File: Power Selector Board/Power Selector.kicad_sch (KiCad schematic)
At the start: 23 parts, among them J101 MSD-DB01M-12P, J102 MSD-DB01F-12P_1, J103 64900221122, J104 64900221122, J105 64900221122, K101 G6SK-2G DC24, U101 1720466, U102 LMW78_24-0.3RL, U103 LMW78_24-0.3RL

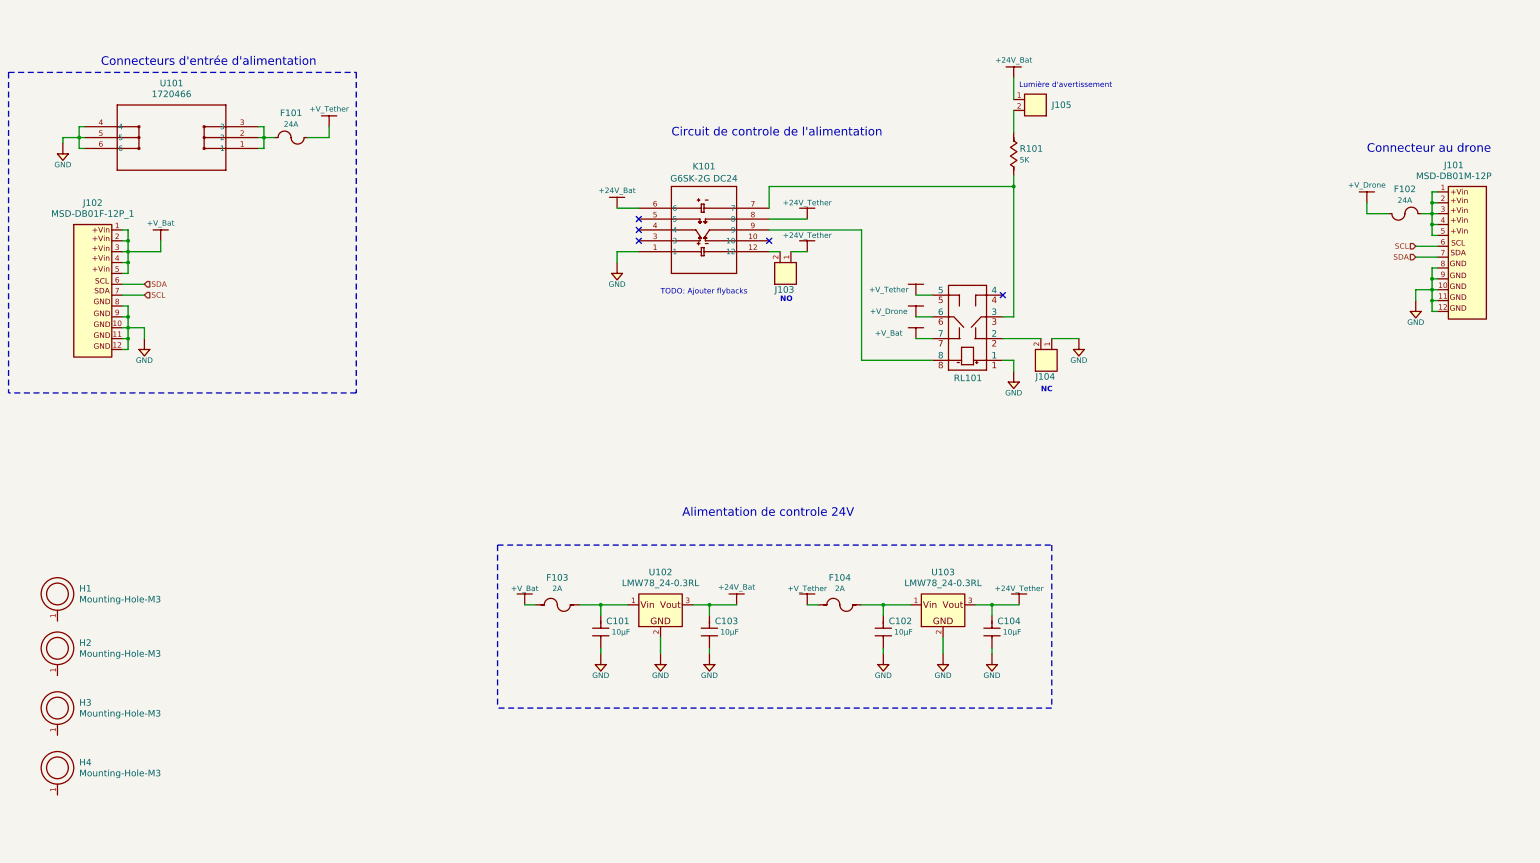
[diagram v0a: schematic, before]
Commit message: Fix du bug github, devrait etre la bonne version
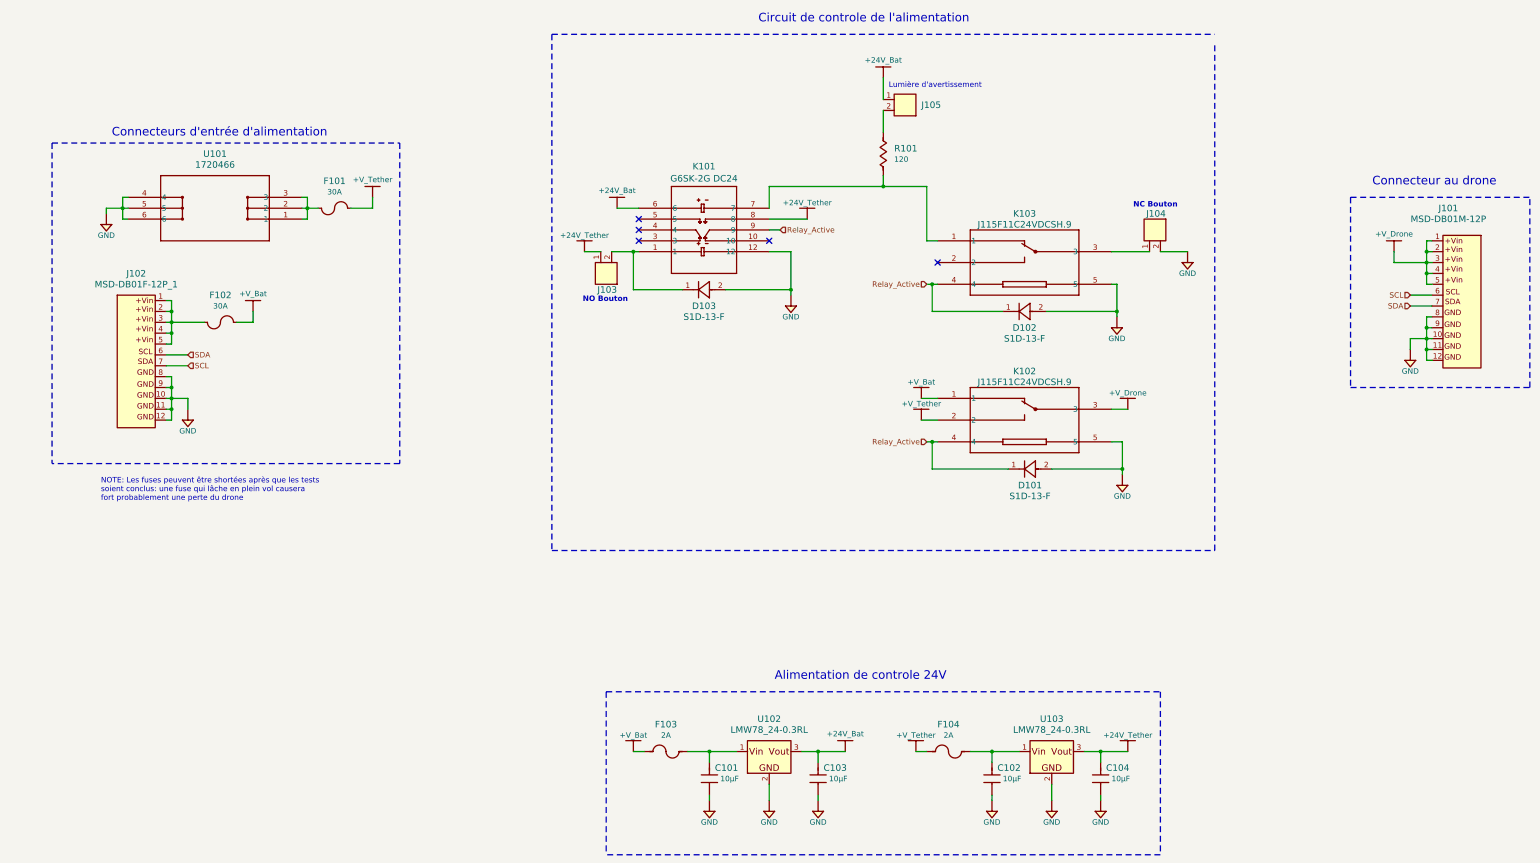
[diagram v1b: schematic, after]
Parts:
- removed H1, H2, H3, H4: Mounting-Hole-M3, Connectors:Mounting_Hole_3mm, symbol Mechanicals:Mounting-Hole-M3
- removed RL101: 2-1462039-9, Relays:2-1462039-9, symbol Relays:2-1462039-9
- added D101, D102, D103: S1D-13-F, Diodes:SMA_DIO, symbol Diodes:S1D-13-F
- added K102, K103: J115F11C24VDCSH.9, RELAY5_J115F11C24VDCSH.9_CRS, symbol Relays:J115F11C24VDCSH.9
- F101, F102: Current Rating (A) 24A -> 30A
- J101, J102: footprint Connectors:MSD-DB01F-12P-V2.0 -> Connectors:649012227222
- R101: Resistance (Ohms) 5K -> 120
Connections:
- net GND: now also J104.2, K101.12, D101.2, D102.2, D103.2, K102.5, K103.5; no longer J104.1, K101.1
- net at K101.7, R101.1: now also K103.1
- net at J103.2: now also K101.1, D103.1; no longer K101.12
- net Relay_Active: now reaches K101.9
- net Relay_Active: now also D101.1, D102.1, K102.4, K103.4
- net +V_Drone: now reaches J101.1, J101.2, J101.3, J101.4, J101.5
- net +V_Drone: now also F101.1, F104.1, K102.2, K102.3; no longer F102.~
- net at U101.1, U101.2, U101.3: now also F101.2; no longer F101.~
- net +VBat: no longer names the net of J102.1, J102.2, J102.3, J102.4, J102.5
- net +VBat: now also F102.2; no longer F101.~, F102.~, F103.1, F104.1
- net 24V renamed 24V_Bat
- net 24V_Bat: no longer C104.2, J103.1, K101.8, U103.3 (Vout)
- new net: J104.1, K103.3
- new net +V_Bat: F102.1, F103.1, K102.1
- new net 24V_Tether: C104.2, J103.1, K101.8, U103.3 (Vout)
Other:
- note added: "NC Bouton"
- note added: "NO Bouton"
- note added: "NOTE: Les fuses peuvent être shortées après que les tests soient conclus: une fuse qui lâche en plein vol causera fort probablement une perte du drone"
- note removed: "NC"
- note removed: "NO"
- note removed: "TODO: Ajouter flybacks"
- moved on the sheet: C101, C102, C103, C104, F103, F104, J101, J102, J104, J105, R101, U101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
